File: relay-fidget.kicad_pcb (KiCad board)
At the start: 2 copper layers, 40 x 90 mm, 5 parts

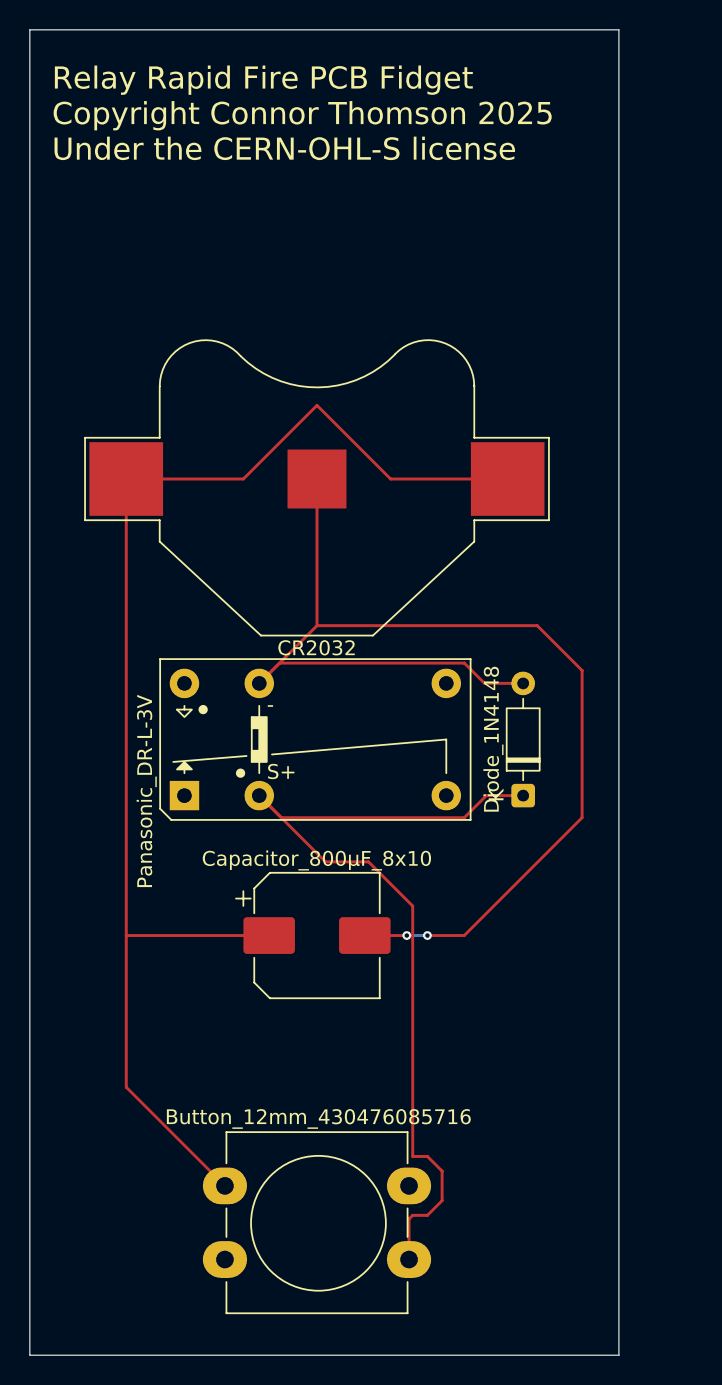
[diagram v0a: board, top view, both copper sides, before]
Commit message: Update relay-fidget.kicad_pcb
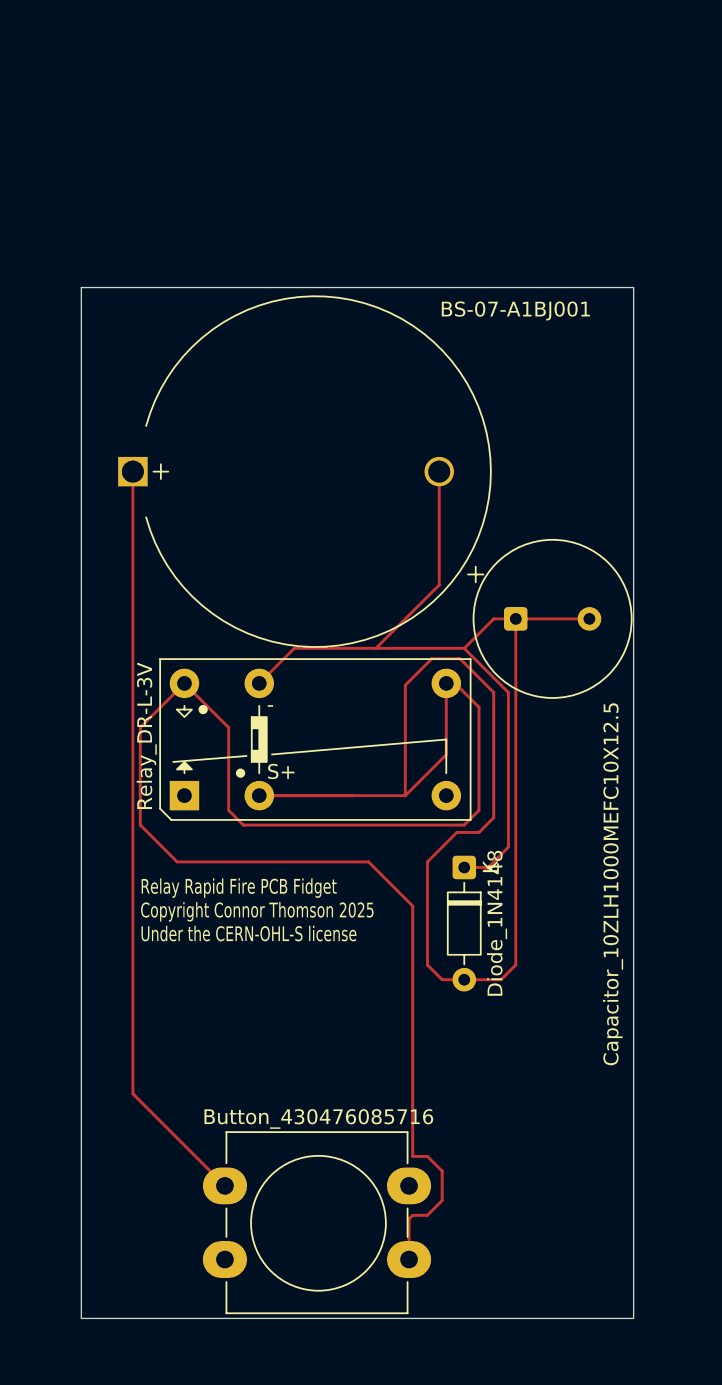
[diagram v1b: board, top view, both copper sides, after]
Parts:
- removed CR2032: CR2032, Battery:BatteryHolder_Multicomp_BC-2001_1x2032
- removed Capacitor_800µF_8x10: Capacitor_800µF_8x10, Capacitor_SMD:CP_Elec_8x10
- added BS-07-A1BJ001: BatteryHolder_MYOUNG_BS-07-A1BJ001_CR2032, Battery:BatteryHolder_MYOUNG_BS-07-A1BJ001_CR2032, F.Cu at (109.5, 85.0)
- added Capacitor_10ZLH1000MEFC10X12.5: Capacitor_10ZLH1000MEFC10X12.5, Capacitor_THT:CP_Radial_Tantal_D10.5mm_P5.00mm, F.Cu at (135.5, 95.0)
- moved Diode_1N4148 6.31 mm to (132.0, 111.9), turned to -90 degrees
- renumbered Button_12mm_430476085716 to Button_430476085716, Panasonic_DR-L-3V to Relay_DR-L-3V
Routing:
- net (no net): track 232.0 -> 296.2 mm, vias 2 -> 0
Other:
- board size 40 x 90 mm -> 37.5 x 70 mm
